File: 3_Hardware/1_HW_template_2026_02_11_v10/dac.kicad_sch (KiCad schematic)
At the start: 4 parts, among them U5 MCP6002-xSN

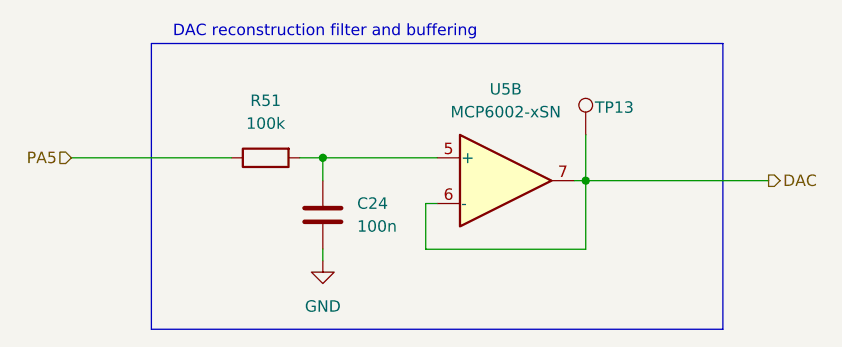
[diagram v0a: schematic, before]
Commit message: layout template
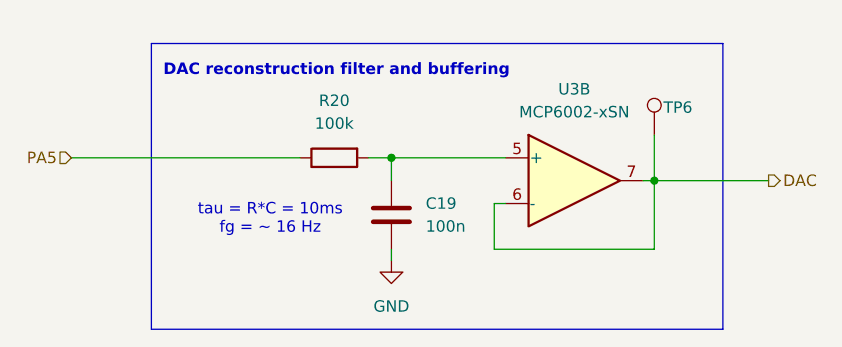
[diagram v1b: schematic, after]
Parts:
- renumbered C24 to C19, R51 to R20, TP13 to TP6, U5 to U3
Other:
- note added: "tau = R*C = 10ms fg = ~ 16 Hz"
- moved on the sheet: C19, R20, TP6, U3B
